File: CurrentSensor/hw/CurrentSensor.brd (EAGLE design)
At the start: 52 x 50 mm, 45 parts, among them IC1 LM317, IC2 74HC595, IC3 ATTINY45, X1 VCC_IN, X2 CHARGE_IN, X3 GND_TO_ACC, X4 GND_FROM_CHARGE

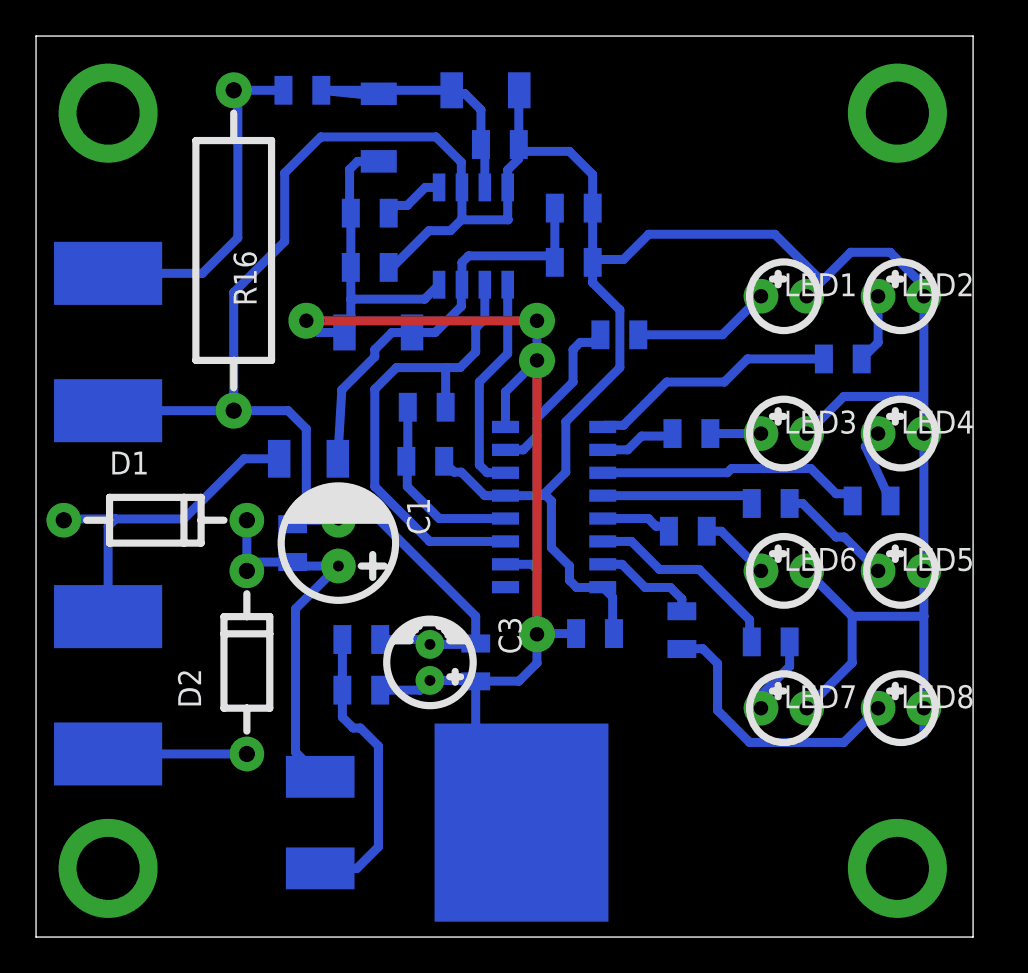
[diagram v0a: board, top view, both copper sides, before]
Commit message: Curent sensor. Routed.
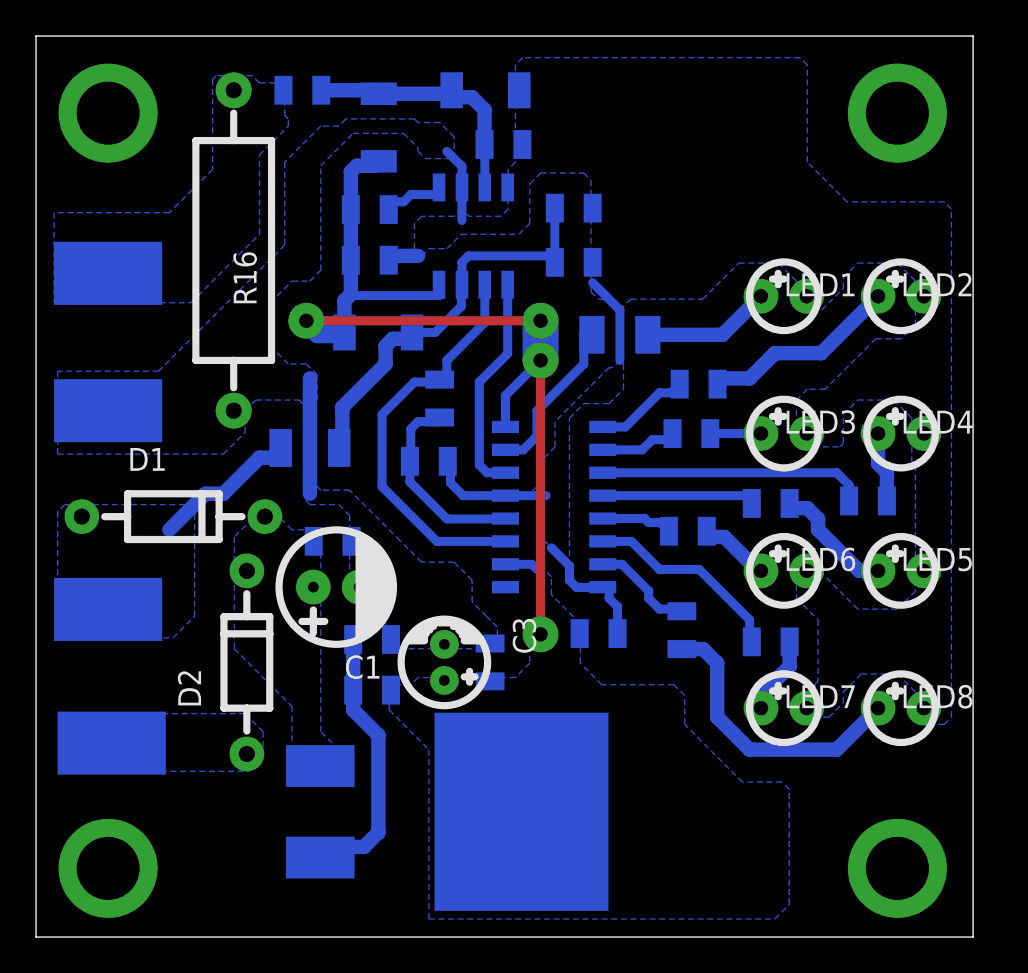
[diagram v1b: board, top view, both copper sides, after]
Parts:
- R1: device __MyCommonLib1:RSMD_0805 -> __MyCommonLib1:RSMD_1206
- moved R2 8.12 mm to (39.8, 30.7)
- moved C1 2.44 mm to (19.7, 19.4), turned to 180 degrees
- moved C2 2.22 mm to (19.5, 22.0), turned to 180 degrees
- moved D1 1.02 mm to (10.6, 23.3)
- moved R6 0.87 mm to (25.4, 29.9), turned to 270 degrees
- moved C3 0.80 mm to (25.7, 15.2)
- moved C4 0.80 mm to (28.2, 15.2)
- moved X2 0.63 mm to (4.20, 10.8)
- moved R12 0.61 mm to (18.2, 27.1)
- moved IC1 0.60 mm to (29.9, 6.95)
- moved R3 0.60 mm to (21.6, 13.7)
- moved R8 0.60 mm to (21.6, 16.5)
- moved C9 0.40 mm to (21.5, 37.6)
- moved X1 0.40 mm to (4.00, 18.2)
- moved C8 0.20 mm to (28.9, 44.0)
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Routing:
- net GND: track 190.7 -> 31.5 mm
- net +5V: track 80.9 -> 59.0 mm
- net N$17: track 21.4 -> 0.00 mm
- net N$36: track 19.1 -> 0.00 mm
- net N$37: track 19.0 -> 8.37 mm
- net N$31: track 13.8 -> 5.26 mm
- net N$38: track 7.70 -> 0.00 mm
- net N$24: track 3.86 -> 10.9 mm
- net LED_SCK: track 26.5 -> 22.4 mm
- net I_SHUNT_ADC: track 16.9 -> 14.1 mm
- net N$39: track 16.3 -> 15.1 mm
- net VOLTAGE_ADC: track 23.7 -> 23.0 mm
- net N$23: track 15.4 -> 15.9 mm
- net N$19: track 7.70 -> 7.17 mm
- added copper zone on layer 16, net +5V
- added copper zone on layer 16, net GND
- added copper zone on layer 16, net N$17
- added copper zone on layer 16, net N$36
- added copper zone on layer 16, net N$37
- added copper zone on layer 16, net N$38
